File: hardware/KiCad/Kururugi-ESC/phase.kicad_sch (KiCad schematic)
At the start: 21 parts, among them J9 Conn_01x01, Q1 CSD18540Q5B, Q2 CSD18540Q5B, U4 2EDL8024

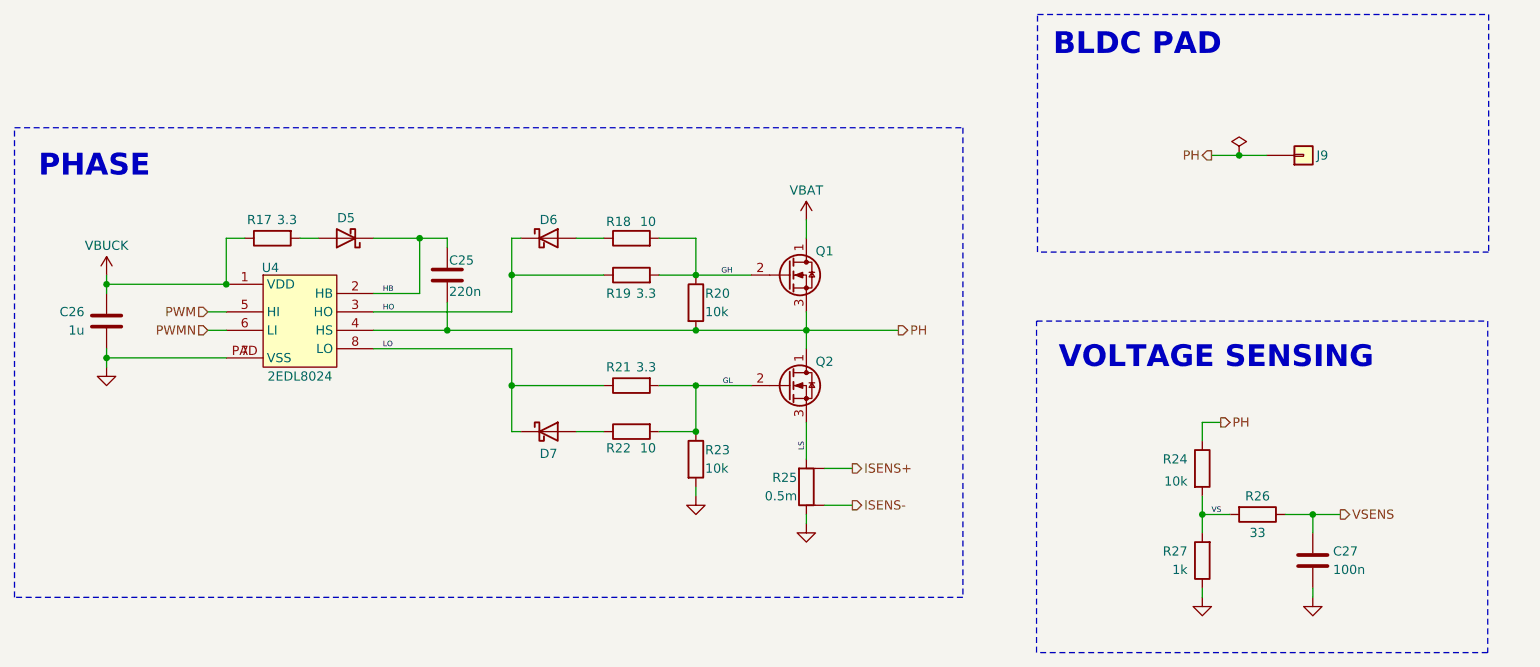
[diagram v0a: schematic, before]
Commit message: Kicad minor corrections
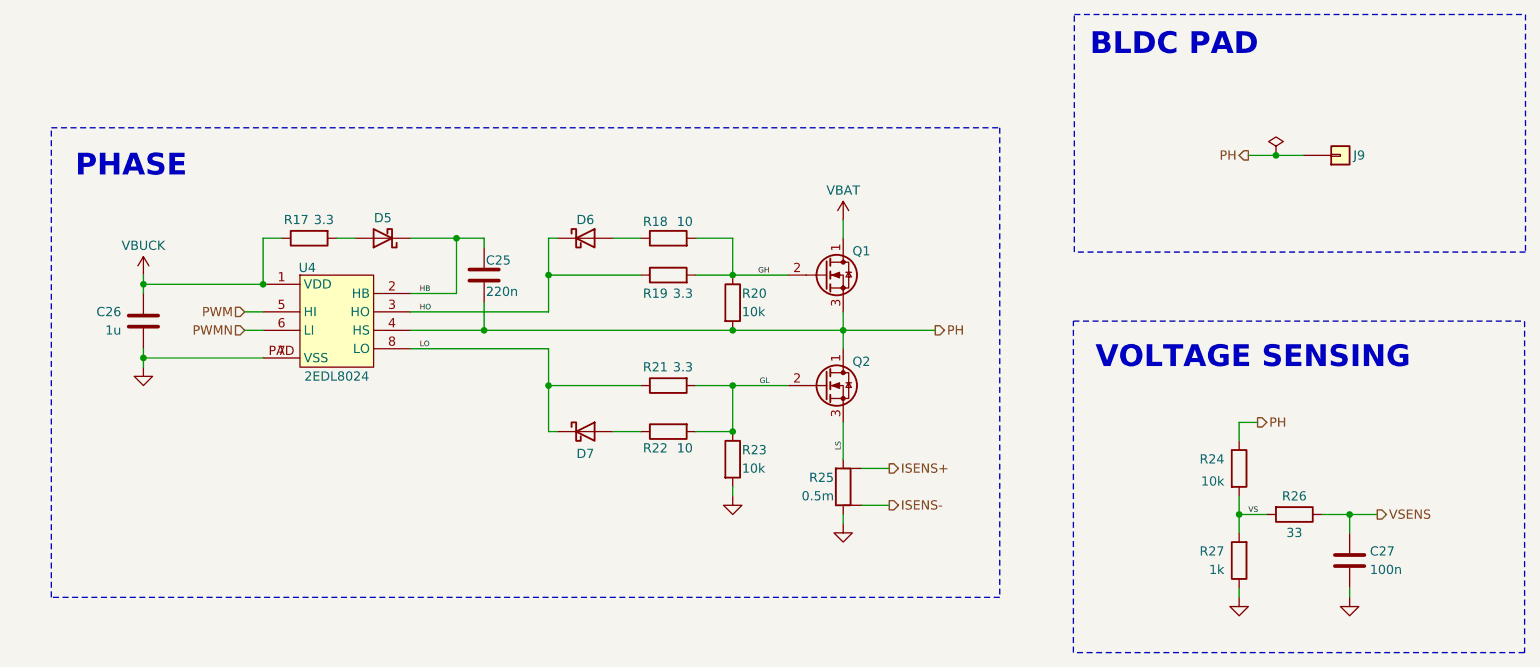
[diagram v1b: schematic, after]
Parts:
- R26: LCSC C25752 -> C25105
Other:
- moved on the sheet: C25, C26, C27, D5, D6, D7, J9, Q1, Q2, R17, R18, R19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
